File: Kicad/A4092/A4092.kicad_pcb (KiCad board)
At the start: 4 copper layers, 175.6 x 122.1 mm, 127 parts, among them CN1 Zorro3, J1 5749721-7, J2 5749721-7, J3 TO-LED, J4 TO-MB, J5 TO-A3000-LED, J6 TO-A3000-MB, J8 Conn_01x06_Pin, U1 SN74ABT16543DGGR, U10 DS21S07A, U11 DS21S07A, U12 DS21S07A, U13 W25X40CLSN, U2 SN74ABT16543DGGR, U3 SN74ABT16543DGGR, U4 SN74ABT16543DGGR, U5 74LVC07APW_118, U6 SN74ABT16245ADGGR, U7 AMS1117-3.3, U8 XC95144XL-TQ144, U9 LSI53C770 SCSI Host Controller, Y1 Abracon ACO-50MHz, Y2 Abracon ACO-40MHz

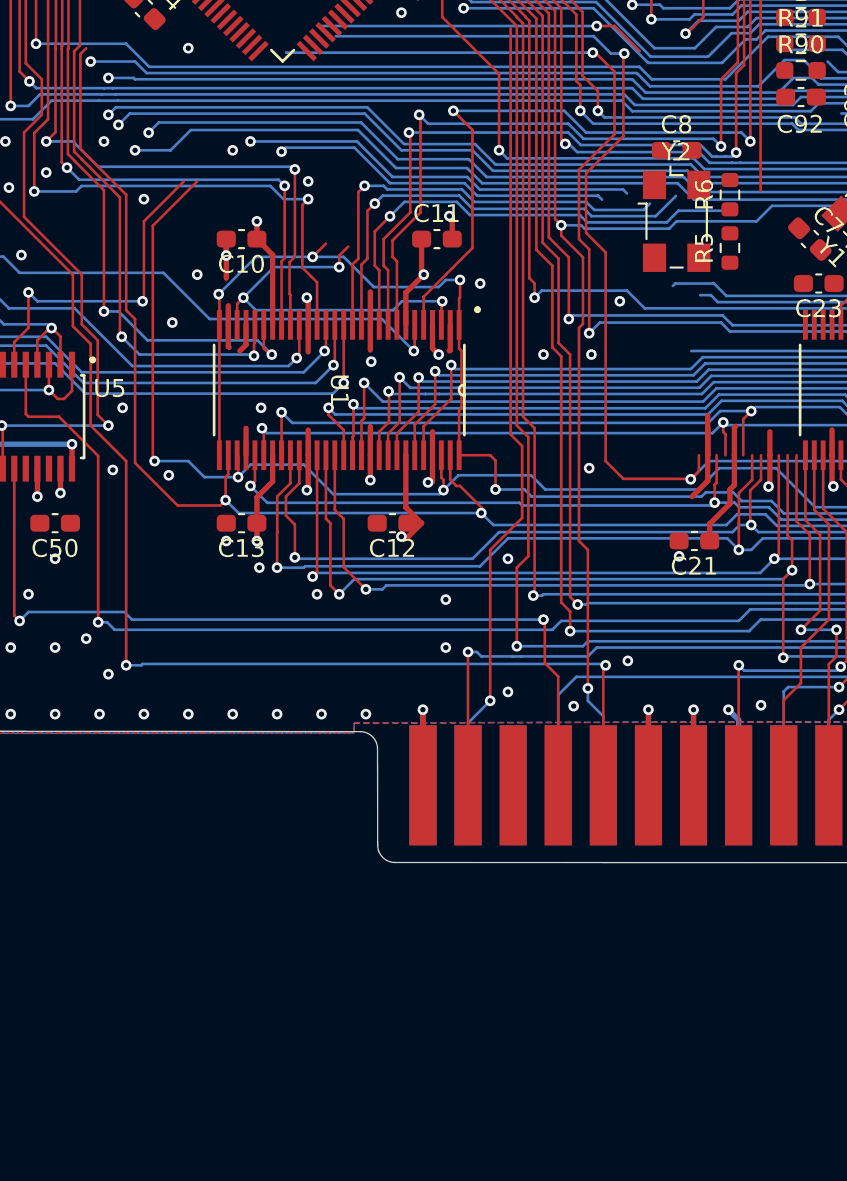
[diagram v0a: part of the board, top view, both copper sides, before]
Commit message: Update PCB from Schematic
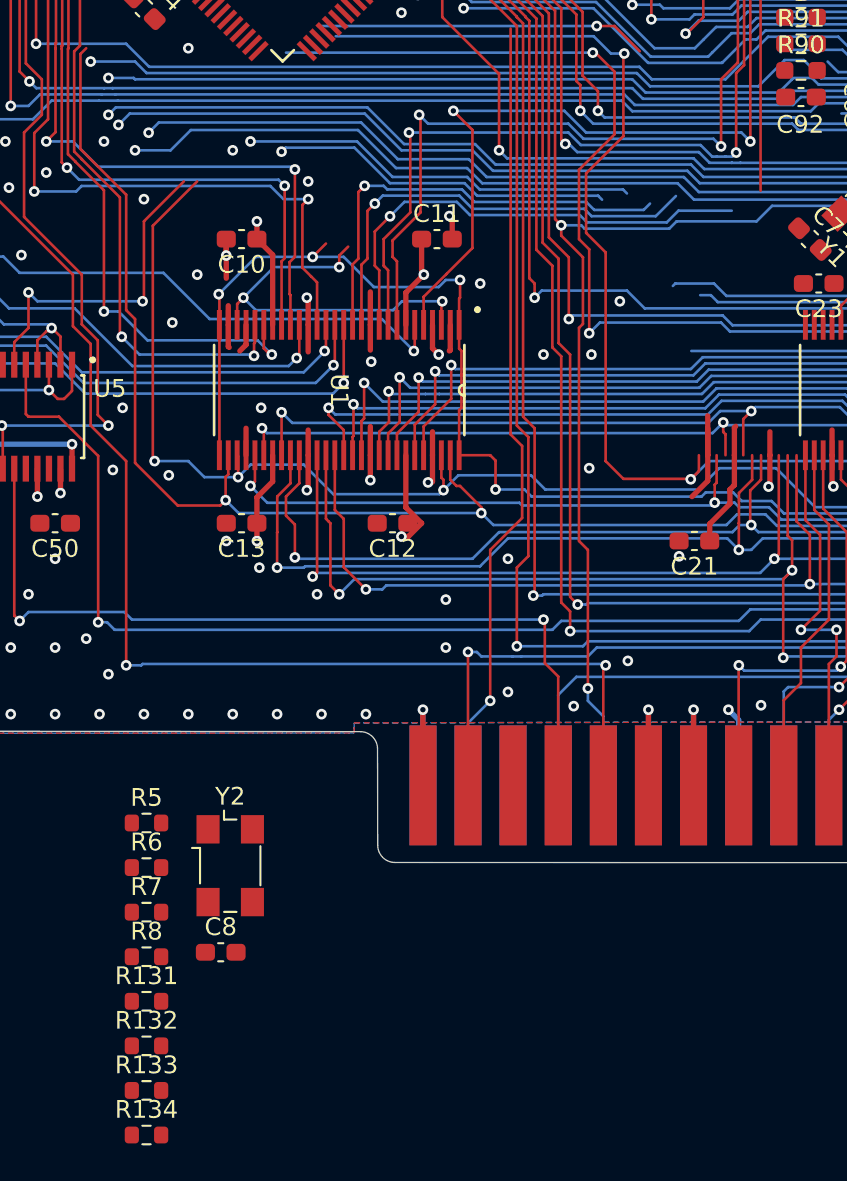
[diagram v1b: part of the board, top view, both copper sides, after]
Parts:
- added R131: 33, Resistor_SMD:R_0603_1608Metric, F.Cu at (80.1, 162.4)
- added R132: 33, Resistor_SMD:R_0603_1608Metric, F.Cu at (80.1, 164.9)
- added R133: 33, Resistor_SMD:R_0603_1608Metric, F.Cu at (80.1, 167.4)
- added R134: 33, Resistor_SMD:R_0603_1608Metric, F.Cu at (80.1, 169.9)
- added R7: 0, Resistor_SMD:R_0603_1608Metric, F.Cu at (80.1, 157.4)
- added R8: 22, Resistor_SMD:R_0603_1608Metric, F.Cu at (80.1, 159.9)
- moved C8 51.9 mm to (84.3, 159.7)
- moved R6 50.2 mm to (80.1, 154.9), turned to 0 degrees
- moved R5 46.1 mm to (80.1, 152.4), turned to 0 degrees
- moved Y2 44.1 mm to (84.9, 154.8)
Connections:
- R130 pad 1: SPI_CS_n -> Net-(U13-~{CS})
- R4 pad 2: BCLK -> BCLK_FULL
- U13 pad 1: SPI_CS_n -> Net-(U13-~{CS})
- U13 pad 2: SPI_MISO -> Net-(U13-DO/IO_{1})
- U13 pad 5: SPI_MOSI -> Net-(U13-DI/IO_{0})
- U13 pad 6: SPI_CLK -> Net-(U13-CLK)
- U8 pad 30: BCLK -> BCLK_FULL
- U8 pad 49: PLD_SID -> unconnected-(U8-P49-Pad49)
- U8 pad 91: unconnected-(U8-P91-Pad91) -> BCLK_HALF
- U9 pad 119: (no net) -> GND
